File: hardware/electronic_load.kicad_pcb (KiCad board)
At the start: 2 copper layers, 76.8 x 61 mm, 85 parts, among them J1 Screw_Terminal_01x02, J2 SPI, J3 UART, P1 Power connector, P2 LCD, P3 One Wire, P4 Gate Drain Source, SW1 Reset, SW2 Back, SW3 Down, SW4 Up, SW5 Enter, U1 FDV303N, U2 TLV1117-33, U3 LM358, U4 MCP6002-xSN, U5 ATmega1284P-AU, U6 FDV303N, U7 FDV303N, U8 FDV303N, Y1 16MHz

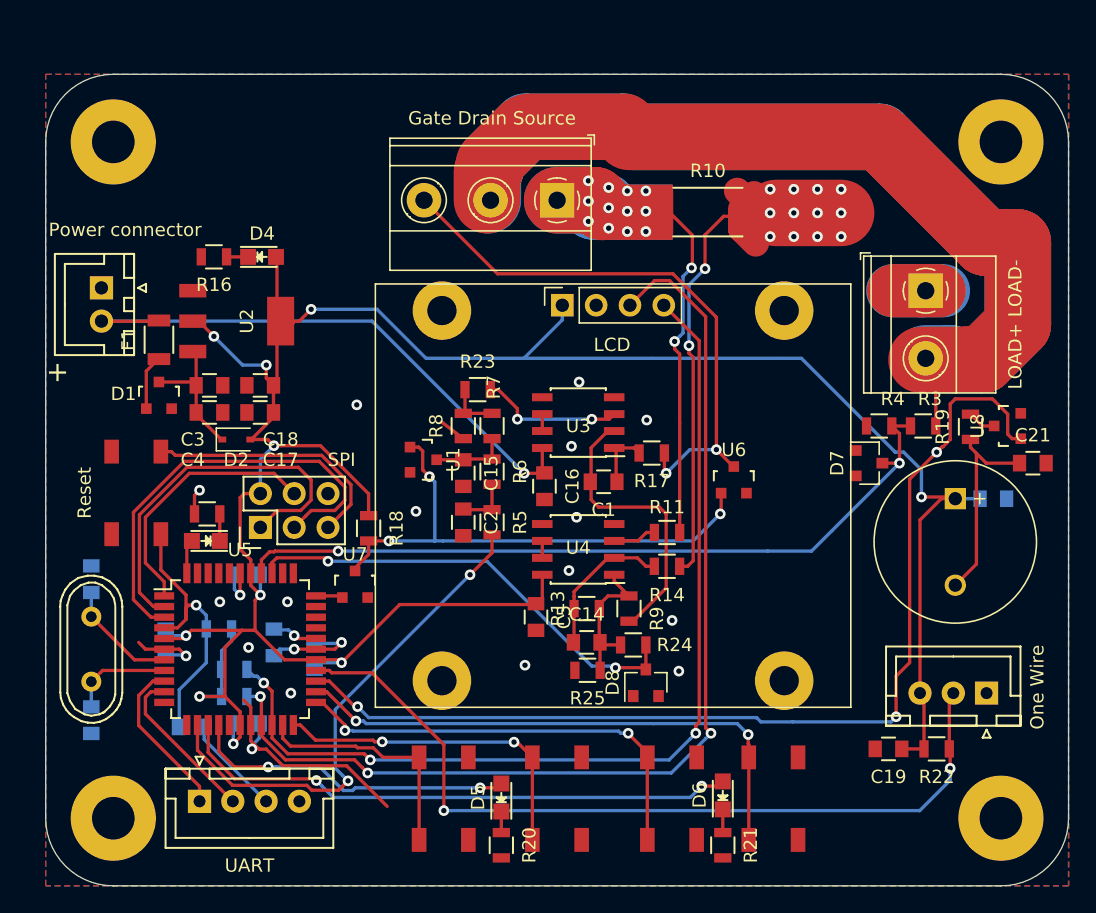
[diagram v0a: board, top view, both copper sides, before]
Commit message: Blebleble
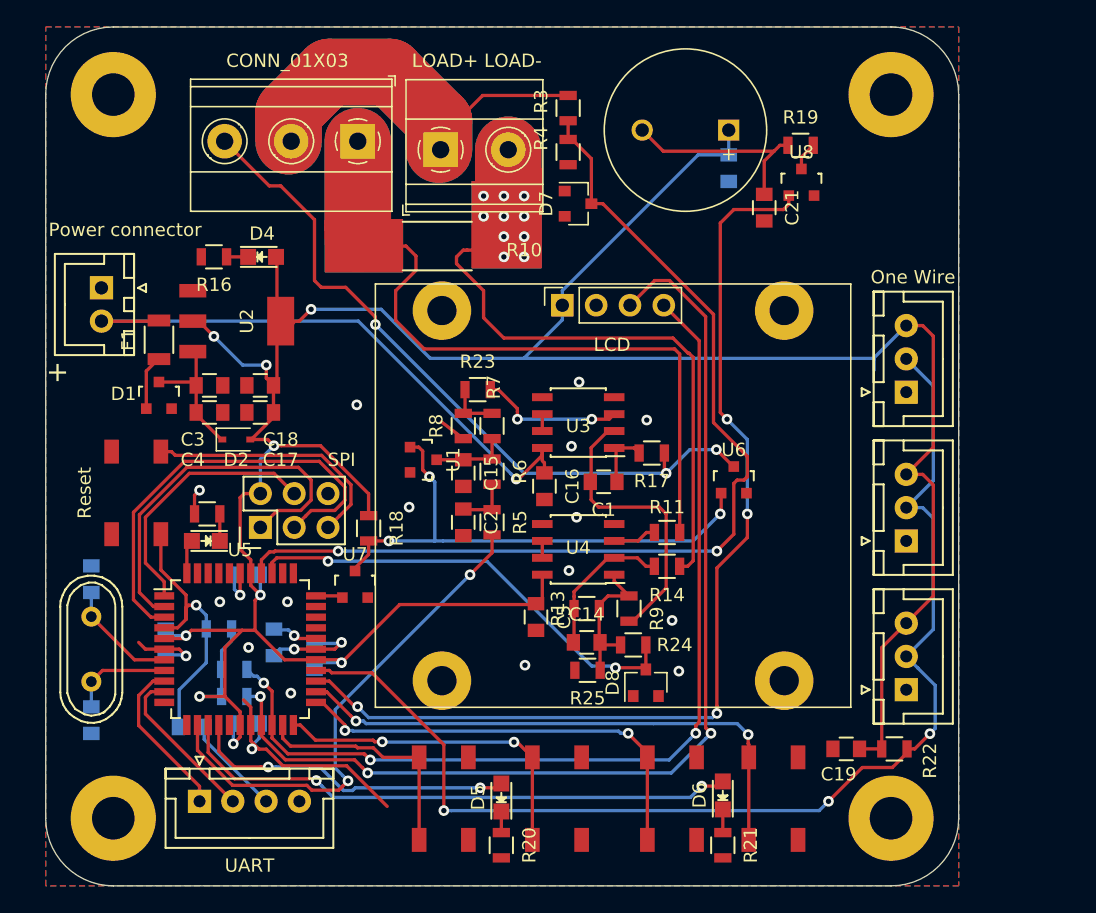
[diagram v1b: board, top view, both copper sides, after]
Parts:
- added P5: One Wire, Connectors_JST:JST_XH_B03B-XH-A_03x2.50mm_Straight, F.Cu at (111.0, 106.2)
- added P6: One Wire, Connectors_JST:JST_XH_B03B-XH-A_03x2.50mm_Straight, F.Cu at (111.0, 117.3)
- P4: value Gate Drain Source -> CONN_01X03
- moved J1 37.9 mm to (76.0, 76.8), turned to 0 degrees
- moved R3 35.8 mm to (85.6, 73.7), turned to 270 degrees
- moved LS1 32.5 mm to (97.7, 75.3), turned to 180 degrees
- moved C20 31.8 mm to (97.7, 78.2), turned to 270 degrees
- moved R4 31.1 mm to (85.6, 77.0), turned to 270 degrees
- moved D7 29.3 mm to (86.3, 80.8)
- moved C21 27.8 mm to (100.3, 81.1), turned to 270 degrees
- moved R19 24.7 mm to (103.1, 76.5), turned to 0 degrees
- moved U8 24.0 mm to (103.1, 79.2), turned to 0 degrees
- moved P3 23.4 mm to (111.0, 95.0), turned to 90 degrees
- moved R10 20.5 mm to (75.8, 84.0)
- moved P4 15.6 mm to (69.8, 76.1)
- moved H6 8.99 mm to (109.9, 72.6)
- moved H8 8.25 mm to (109.9, 127.0)
- moved H5 3.56 mm to (51.4, 72.6)
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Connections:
- J1 pad 1: GND -> /Variable Load/Vload
- J1 pad 2: /Variable Load/Vload -> GND
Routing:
- net /Variable Load/Vload: track 128.1 -> 47.3 mm
- net 3.3V: track 199.9 -> 227.2 mm, vias 10 -> 9
- net ONE_WIRE: track 62.5 -> 89.3 mm, vias 2 -> 3
- net /Variable Load/Current_feedback_P: track 39.7 -> 61.3 mm, vias 12 -> 0
- net VOLTAGE_SENSE: track 57.4 -> 75.4 mm
- net (no net): track 28.3 -> 39.9 mm, vias 4 -> 2
- net Net-(P4-Pad3): track 43.5 -> 54.4 mm, vias 2 -> 3
- net GND: track 59.9 -> 52.1 mm, vias 32 -> 28
- net SPEAKER_DRIVE: track 78.3 -> 76.4 mm, vias 3 -> 4
- net 12V: track 44.3 -> 45.2 mm
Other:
- board size 76.8 x 61 mm -> 68.6 x 64.5 mm
